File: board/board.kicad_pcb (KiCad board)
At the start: 2 copper layers, 21 x 13 mm, 1 part

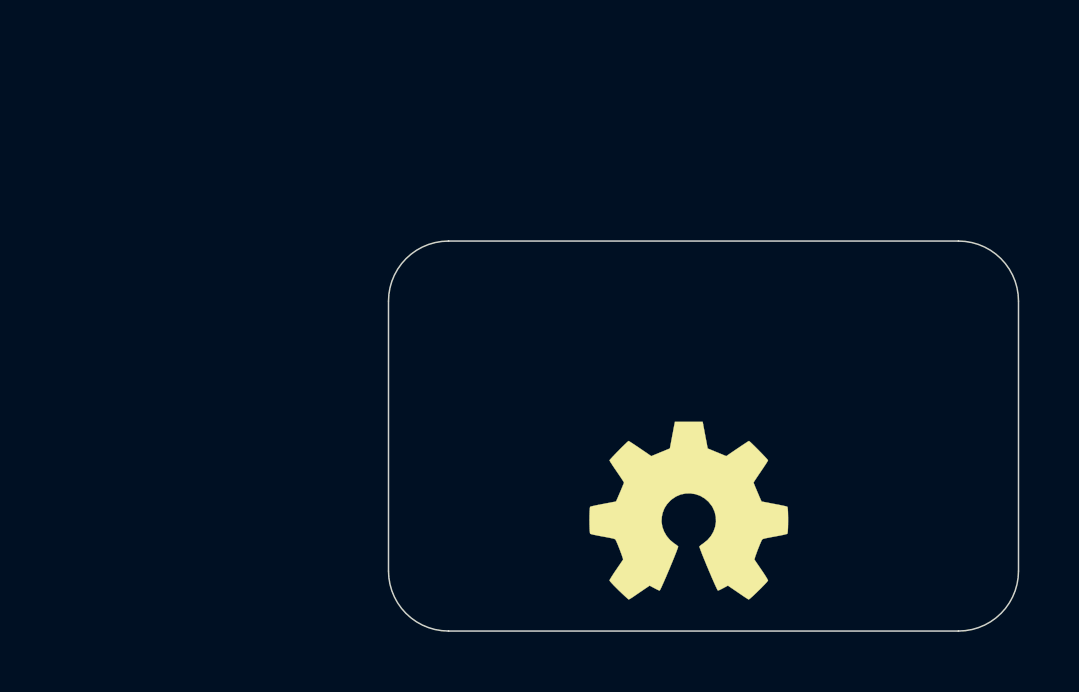
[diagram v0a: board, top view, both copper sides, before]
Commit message: initial
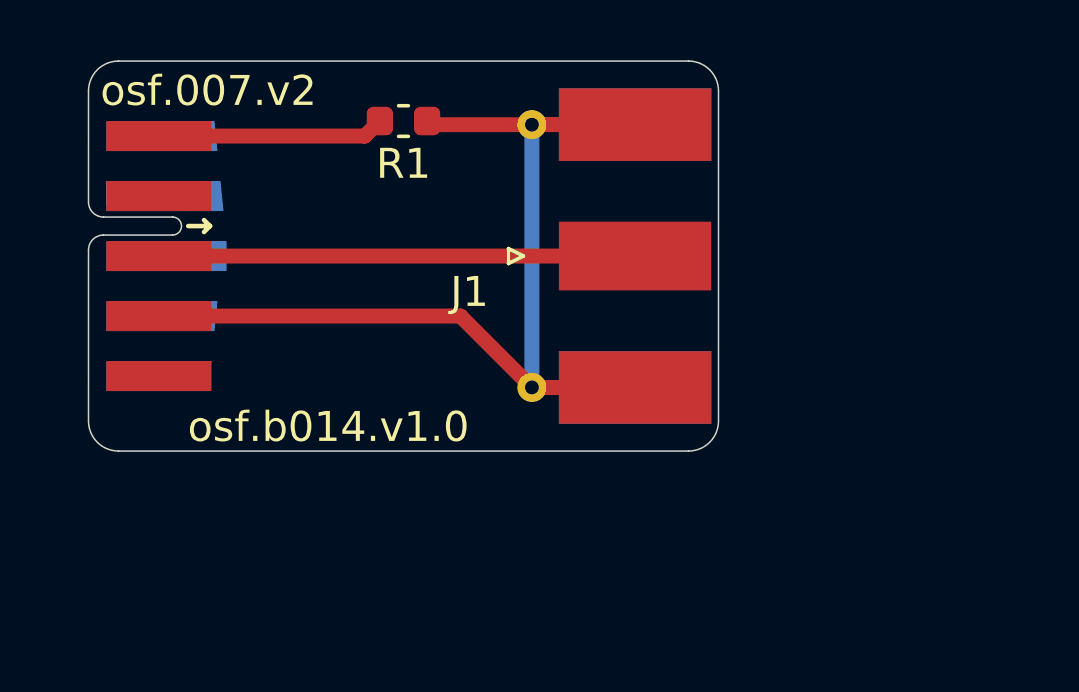
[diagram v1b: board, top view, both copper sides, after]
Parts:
- removed LOGO1: Logo_Open_Hardware_Small, Symbol:OSHW-Symbol_6.7x6mm_SilkScreen
- added J1: Conn_Coaxial, Connector_Coaxial:SMA_Molex_73251-1153_EdgeMount_Horizontal, F.Cu at (146.5, 90.5)
- added J2: 007_ADC_2x2, on_edge:on_edge_2x05_device, F.Cu at (130.0, 90.5)
- added R1: d.n.p, Resistor_SMD:R_0603_1608Metric, F.Cu at (140.5, 86.0)
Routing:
- net Net-(J1-Pad2): track 0.00 -> 32.9 mm
- net Net-(J1-Pad1): track 0.00 -> 14.6 mm
- net GND: track 0.00 -> 7.57 mm
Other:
- outline, holes or cut-outs redrawn
- rule pad_to_mask_clearance: 0 -> 0.051
- board text added: "osf.007.v2"
- board text added: "osf.b014.v1.0"
